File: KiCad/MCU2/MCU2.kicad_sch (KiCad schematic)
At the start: 9 parts, among them J1 Conn_02x03_Counter_Clockwise, J2 Conn_01x06, J3 Conn_01x03, SW1 MCU_Button, U1 ATmega328P-A

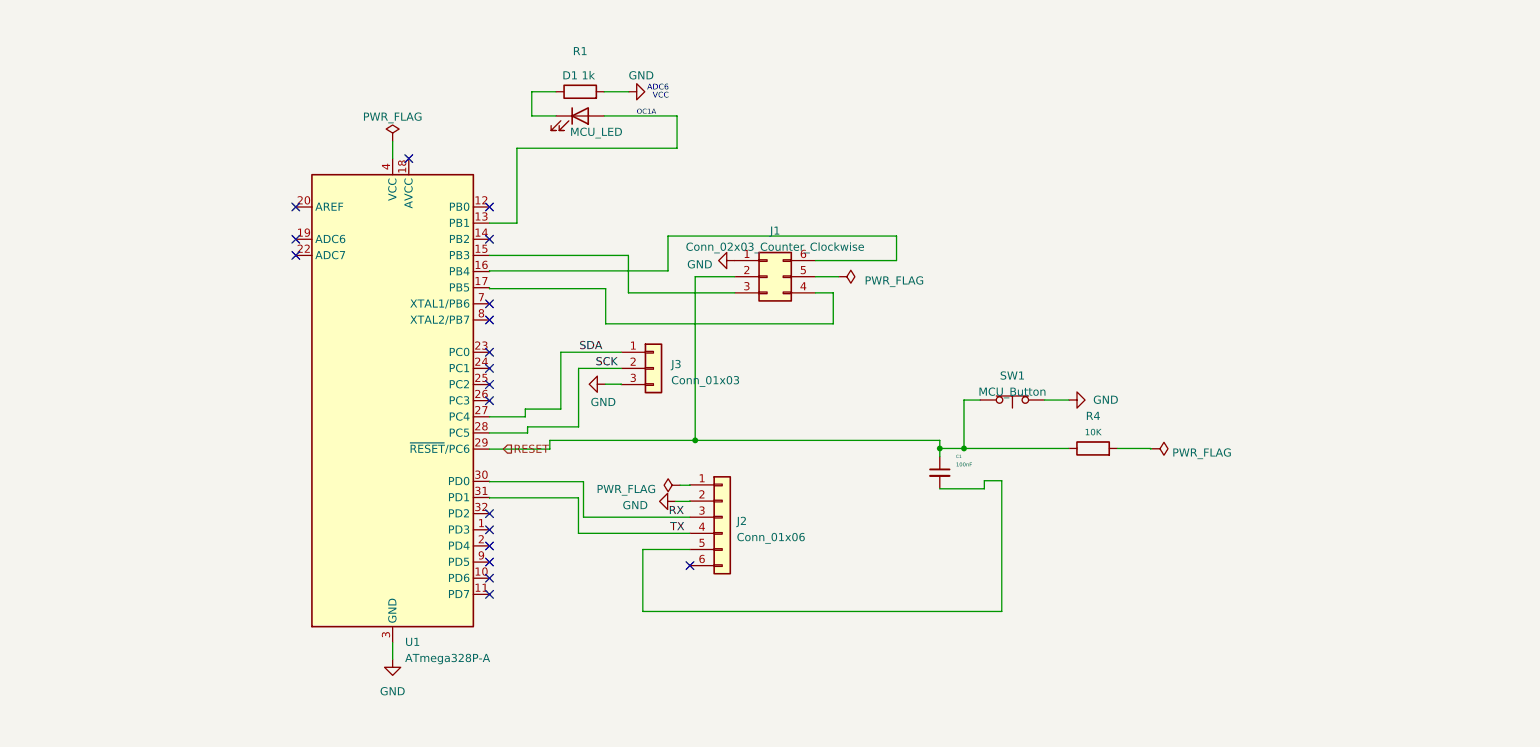
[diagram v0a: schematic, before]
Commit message: update
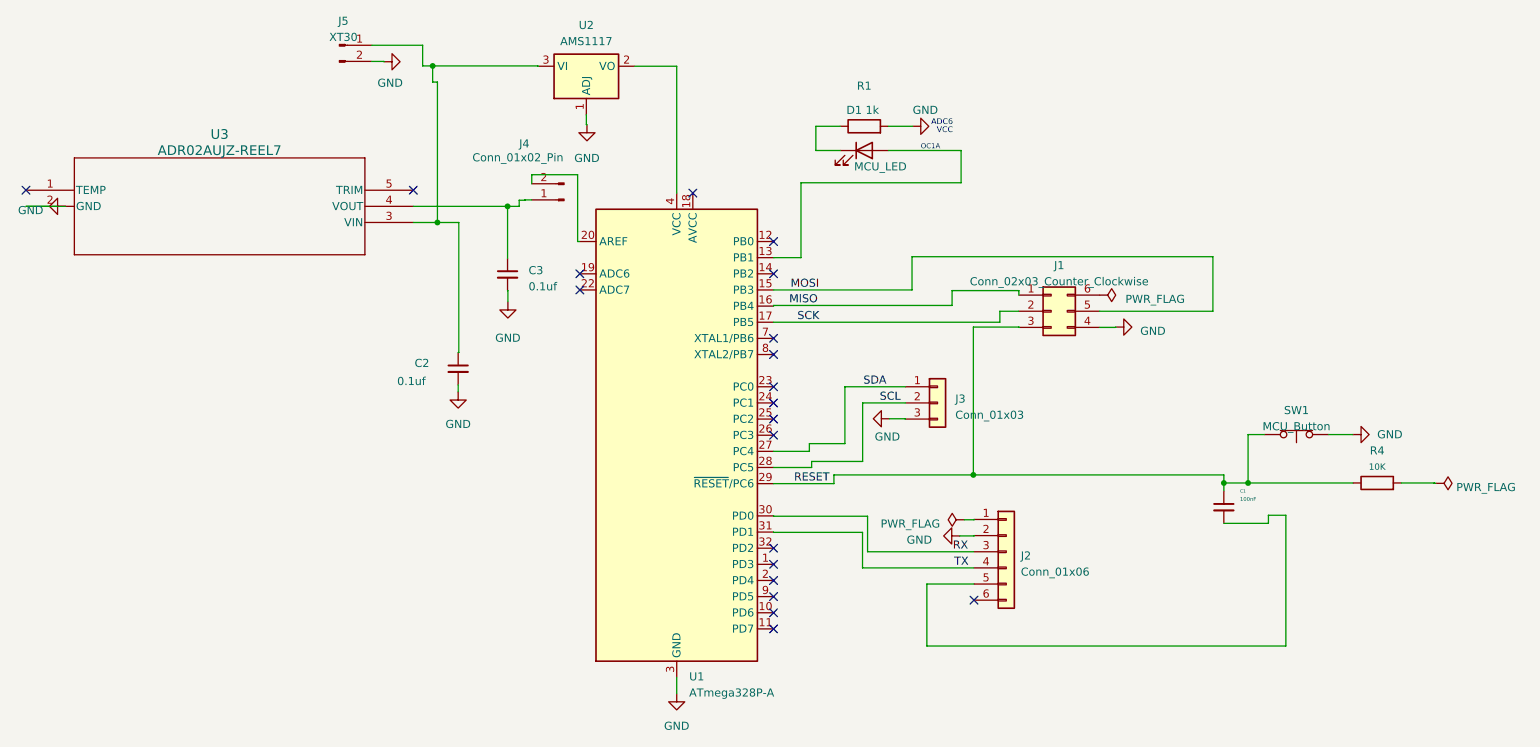
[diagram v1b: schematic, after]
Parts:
- added C2, C3: 0.1uf, Capacitor_SMD:C_1206_3216Metric, symbol Device:C_Small
- added J4: Conn_01x02_Pin, Connector_PinHeader_2.54mm:PinHeader_1x02_P2.54mm_Vertical, symbol Connector:Conn_01x02_Pin
- added J5: XT30, Connector_AMASS:AMASS_XT30U-F_1x02_P5.0mm_Vertical, symbol Connector:Conn_01x02_Pin
- added U2: AMS1117, Package_TO_SOT_SMD:SOT-223-3_TabPin2, symbol Regulator_Linear:AMS1117
- added U3: ADR02AUJZ-REEL7, footprints:UJ_5_ADI, symbol 2023-06-26_00-14-37:ADR02AUJZ-REEL7
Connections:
- net GND: now also J1.4 (Pin_4), C2.2, C3.2, J5.2 (Pin_2), U2.1 (ADJ), U3.2 (GND); no longer J1.1 (Pin_1)
- net RESET: now also J1.3 (Pin_3); no longer J1.2 (Pin_2)
- net SCK: now also J1.2 (Pin_2), U1.17 (PB5); no longer J3.2 (Pin_2), U1.28 (PC5)
- net MOSI: now reaches U1.15 (PB3)
- net MOSI: now also J1.5 (Pin_5); no longer J1.3 (Pin_3)
- net at J1.6 (Pin_6): no longer U1.16 (PB4)
- net at U1.20 (AREF): now also J4.2 (Pin_2)
- net at U1.4 (VCC), U1.6 (VCC): now also U2.2 (VO)
- new net: C2.1, J5.1 (Pin_1), U2.3 (VI), U3.3 (VIN)
- new net: C3.1, J4.1 (Pin_1), U3.4 (VOUT)
- new net MISO: J1.1 (Pin_1), U1.16 (PB4)
- new net SCL: J3.2 (Pin_2), U1.28 (PC5)
- no-connect marks 19 -> 20
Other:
- moved on the sheet: C1, D1, J1, J2, J3, R1, R4, SW1, U1
